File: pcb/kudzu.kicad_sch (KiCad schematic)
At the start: 0 parts

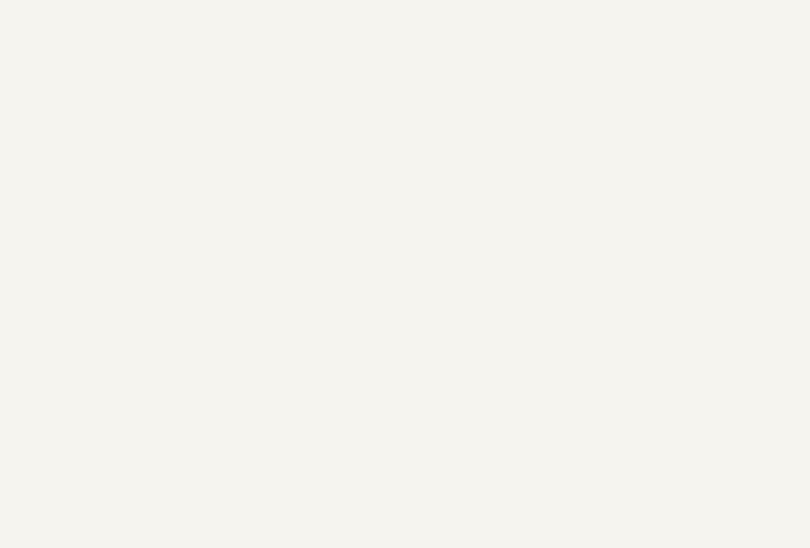
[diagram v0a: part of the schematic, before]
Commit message: pcb: Update schematic to WIP6
Change-Id: I9e9f727ad2774ee986f2f97450dc509901129aec
Reviewed-on: https://pigweed-review.googlesource.com/c/pigweed/kudzu/+/169650
Reviewed-by: Anthony DiGirolamo <tonymd@google.com>
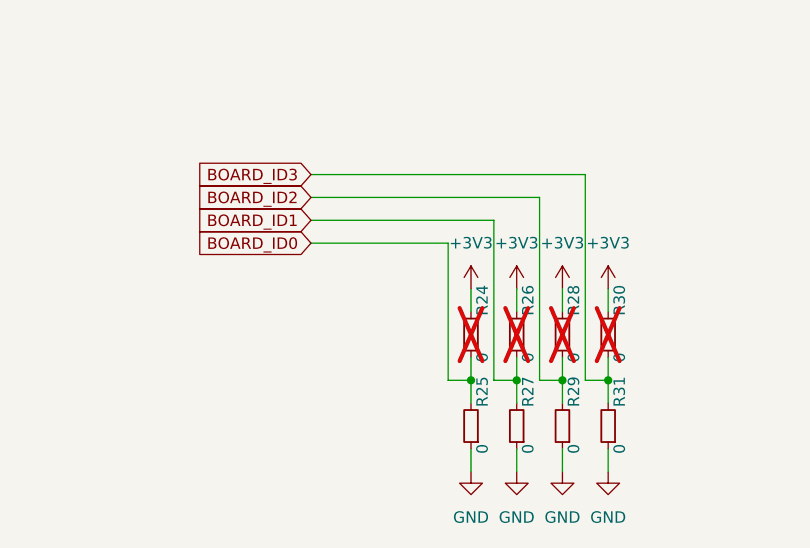
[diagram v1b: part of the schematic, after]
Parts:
- added R24, R25, R26, R27, R28, R29, R30, R31: 0, symbol Device:R_Small
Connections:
- new net +3V3: R24.2, R26.2, R28.2, R30.2
- new net BOARD_ID0: R24.1, R25.2
- new net BOARD_ID1: R26.1, R27.2
- new net BOARD_ID2: R28.1, R29.2
- new net BOARD_ID3: R30.1, R31.2
- new net GND: R25.1, R27.1, R29.1, R31.1
